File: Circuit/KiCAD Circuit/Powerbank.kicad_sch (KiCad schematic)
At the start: 44 parts, among them Q1 NMOS, Q2 PMOS, Q3 NMOS, SW1 SW_Push, SW2 SW_SPST, U1 BQ7692003PW, U2 Arduino_Nano_v3.x

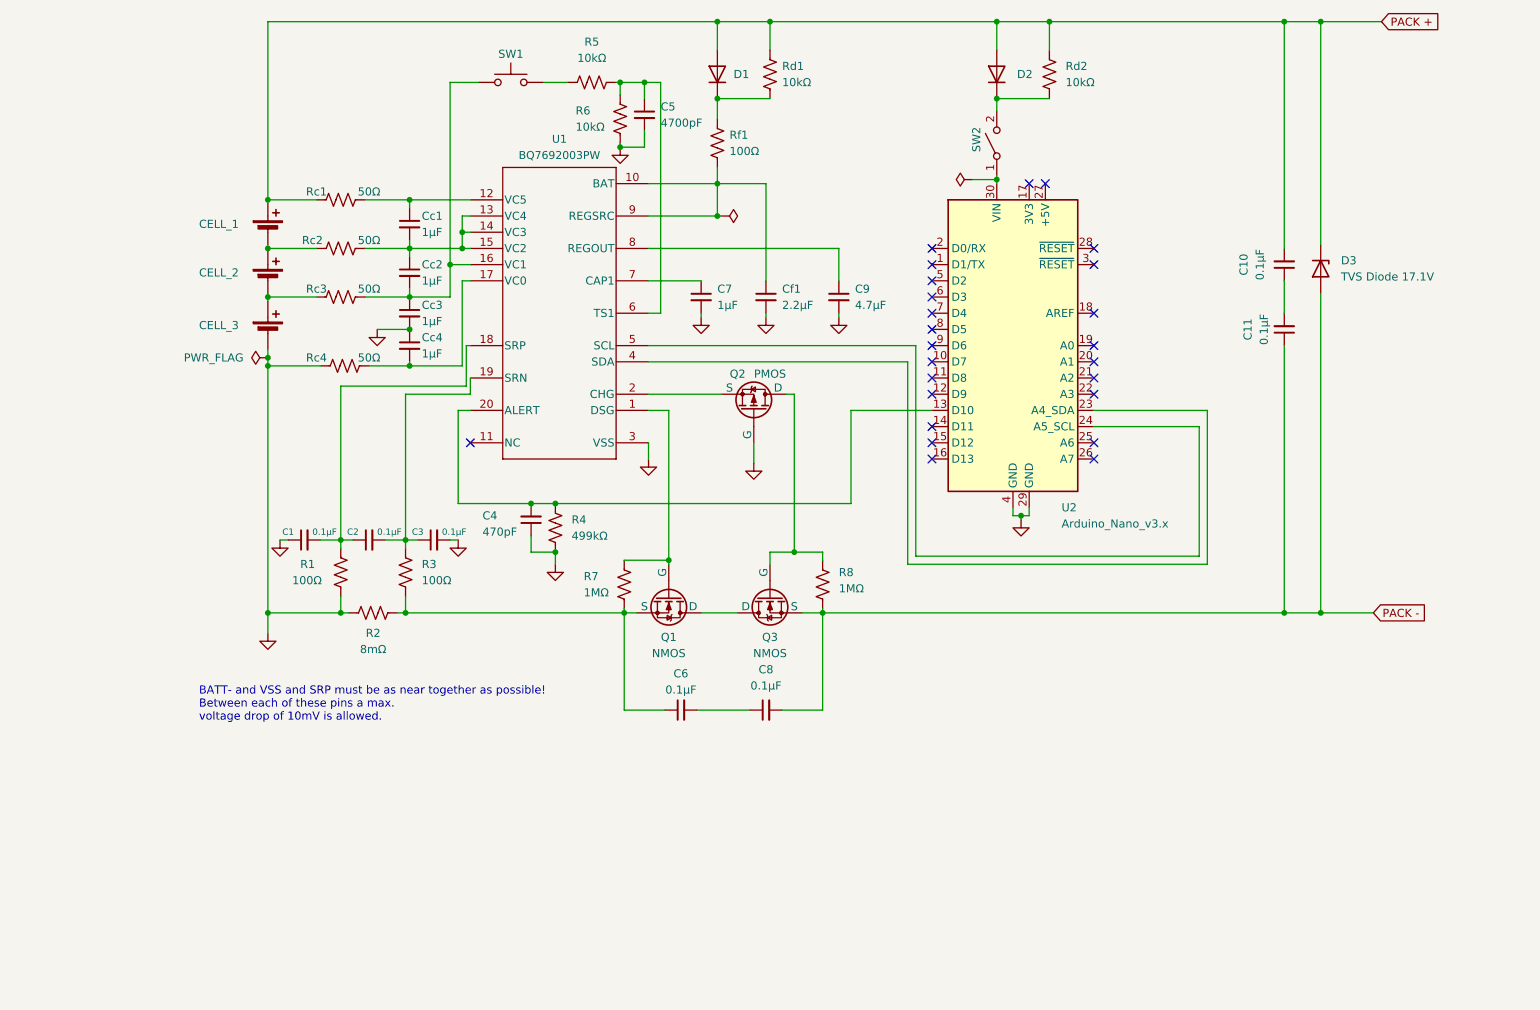
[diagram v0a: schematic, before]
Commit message: Backup
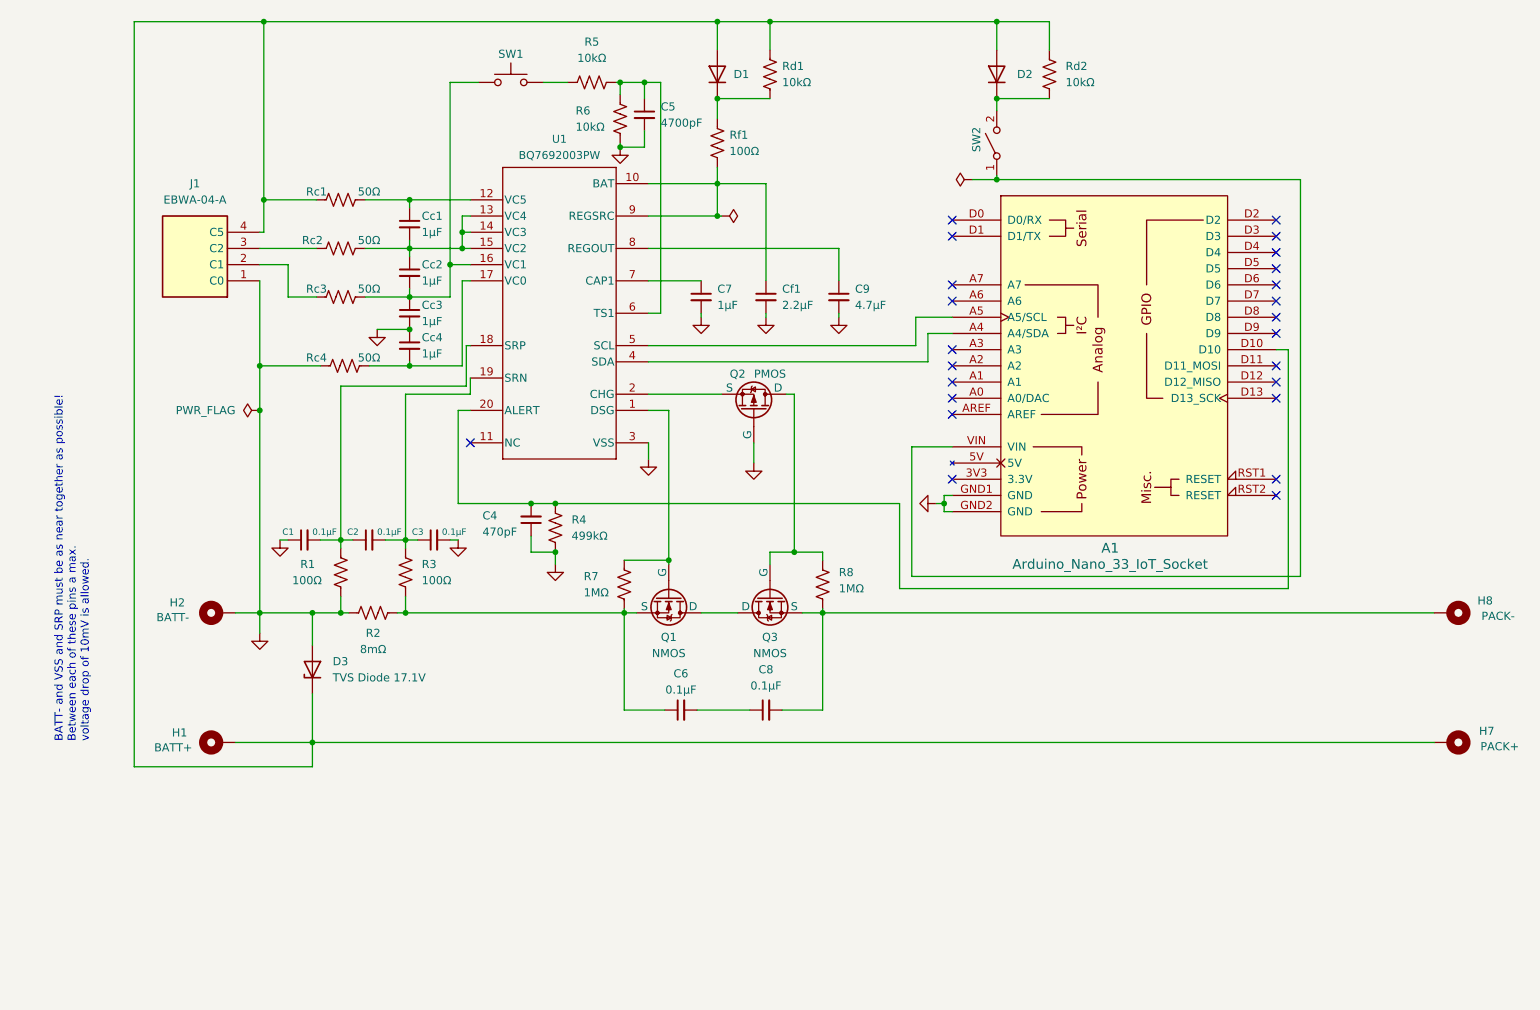
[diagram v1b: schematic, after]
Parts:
- removed C10, C11: 0.1μF, K104K10X7RF53H5:K104K10X7RF53H5_VIS, symbol Device:C_Small
- removed CELL_1, CELL_2, CELL_3: ~, symbol Device:Battery_Cell
- removed U2: Arduino_Nano_v3.x, Arduinos:Arduino_Nano_33_IoT_Socket, symbol MCU_Module:Arduino_Nano_v3.x
- added A1: Arduino_Nano_33_IoT_Socket, Arduinos:Arduino_Nano_33_IoT_Socket, symbol Arduinos:Arduino_Nano_33_IoT_Socket
- added H1: BATT+, Custom Footprints:Power Connection Pads, symbol Mechanical:MountingHole_Pad
- added H2: BATT-, Custom Footprints:Power Connection Pads, symbol Mechanical:MountingHole_Pad
- added H7: PACK+, Custom Footprints:Power Connection Pads, symbol Mechanical:MountingHole_Pad
- added H8: PACK-, Custom Footprints:Power Connection Pads, symbol Mechanical:MountingHole_Pad
- added J1: EBWA-04-A, Custom Footprints:EBWA-04-A, symbol EBWA-04-A:EBWA-04-A
- D1, D2: footprint (none) -> Custom Footprints:1N4149TR; Mouser (none) -> 512-1N4149TR
- Q1, Q3: footprint Custom Footprints:TO-220AB -> Custom Footprints:IRLB4132PBF
- Q2: footprint (none) -> VP3203N3-G:TO-92_MC_MCH; Mouser (none) -> 689-VP3203N3-G
- Rc1, Rc2, Rc3, Rc4: Mouser CMF5550R000FKEK70 -> 71-CMF5550R000FKEK70
- SW1, SW2: footprint Custom Footprints:Push button -> Custom Footprints:Switch Pads
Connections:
- net GND: now also D3.2 (A), A1.GND1 (GND), A1.GND2 (GND), H2.1, J1.1 (C0)
- net at Rc2.1: now also J1.3 (C2)
- net at Rc3.1: now also J1.2 (C1)
- net at C4.2, R4.1, U1.20 (ALERT): now also A1.D10
- net at SW2.1 (A): now also A1.VIN
- net at U1.4 (SDA): now also A1.A4 (A4/SDA)
- net at U1.5 (SCL): now also A1.A5 (A5/SCL)
- net PACK +: no longer names the net of D1.2 (A), D2.2 (A), D3.1 (K), Rc1.1, Rd1.1, Rd2.1
- net PACK +: now also H1.1, H7.1, J1.4 (C5)
- net PACK -: no longer names the net of C8.2, Q3.3 (S), R8.2
- net PACK -: now also H8.1; no longer D3.2 (A)
- no-connect marks 25 -> 24
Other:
- moved on the sheet: D3

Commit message: Backup
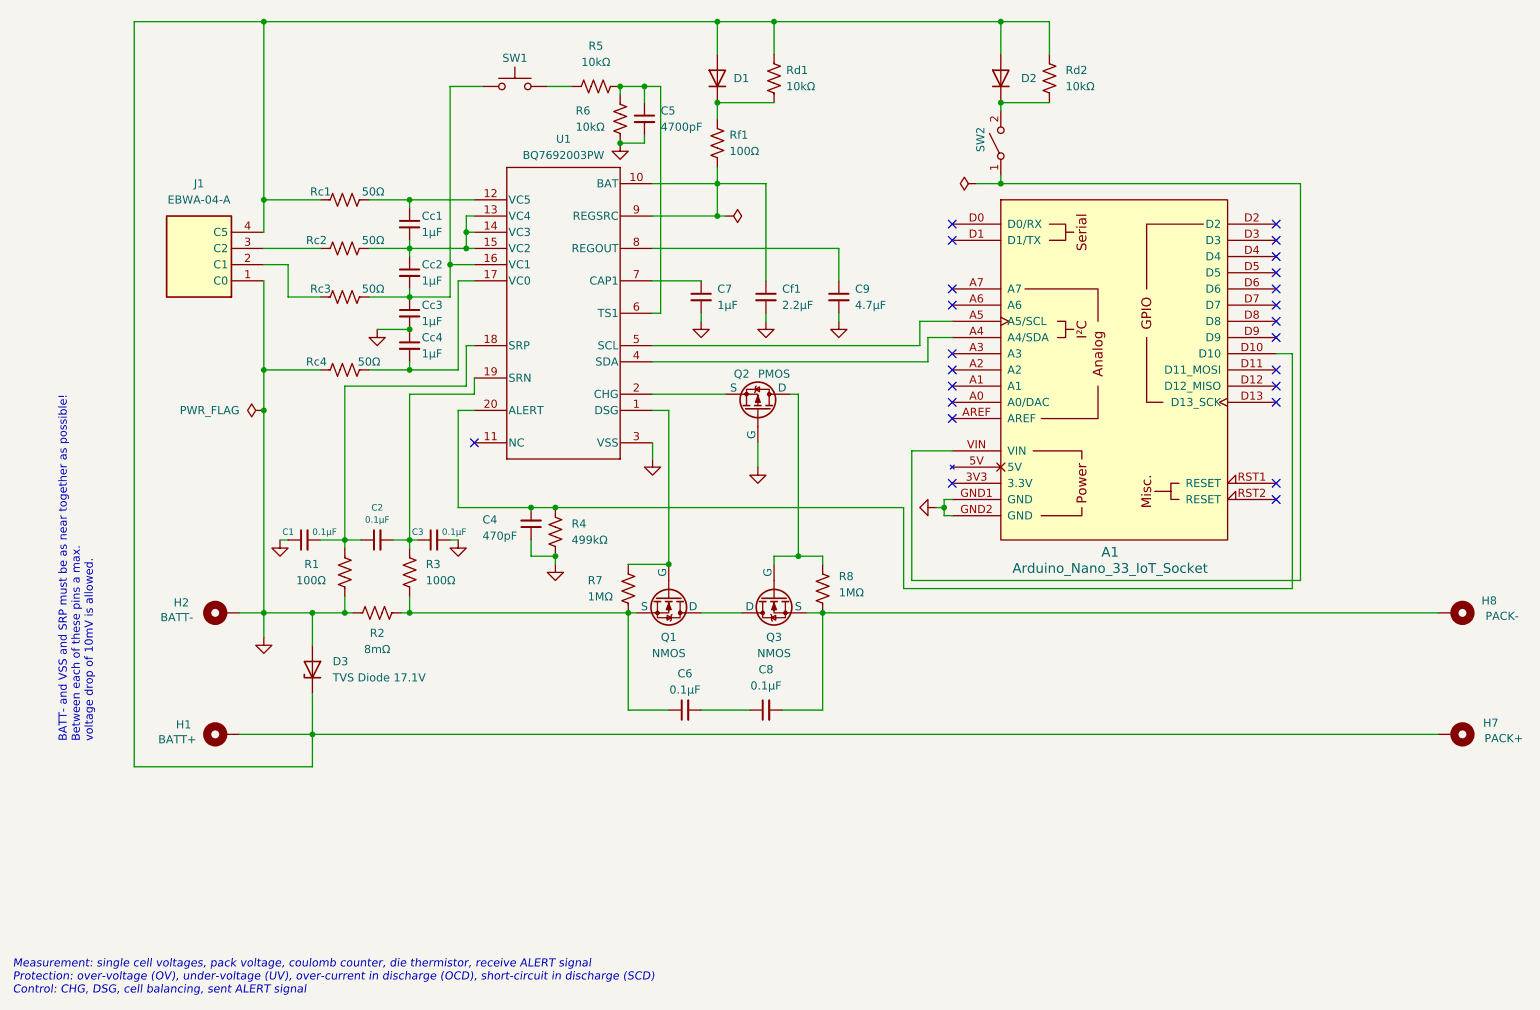
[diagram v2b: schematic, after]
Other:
- note added: "Measurement: single cell voltages, pack voltage, coulomb counter, die thermistor, receive ALERT signal Protection: over-voltage (OV), under-voltage (UV), over-current in discharge (OCD), short-circuit in discharge (SCD) Control: CHG, DSG, cell balancing, sent ALERT signal"
- company: [Private] Léon Becker -> Léon Becker
- title: BQ76920 Power Bank Circuit -> BQ76920 Power Bank Schematic
- moved on the sheet: A1, C2, C4, C5, C6, D1, D2, H1, H2, H7, H8, J1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
